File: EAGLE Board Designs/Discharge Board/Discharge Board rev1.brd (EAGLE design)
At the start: 59 x 77 mm, 25 parts, among them J100 CONNECTOR-2_MICROFIT_SMD_RIGH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, J101 CONNECTOR-2_MICROFIT_SMD_RIGH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, K1 RELAY_SPST_NC_POLARIZED_D_24

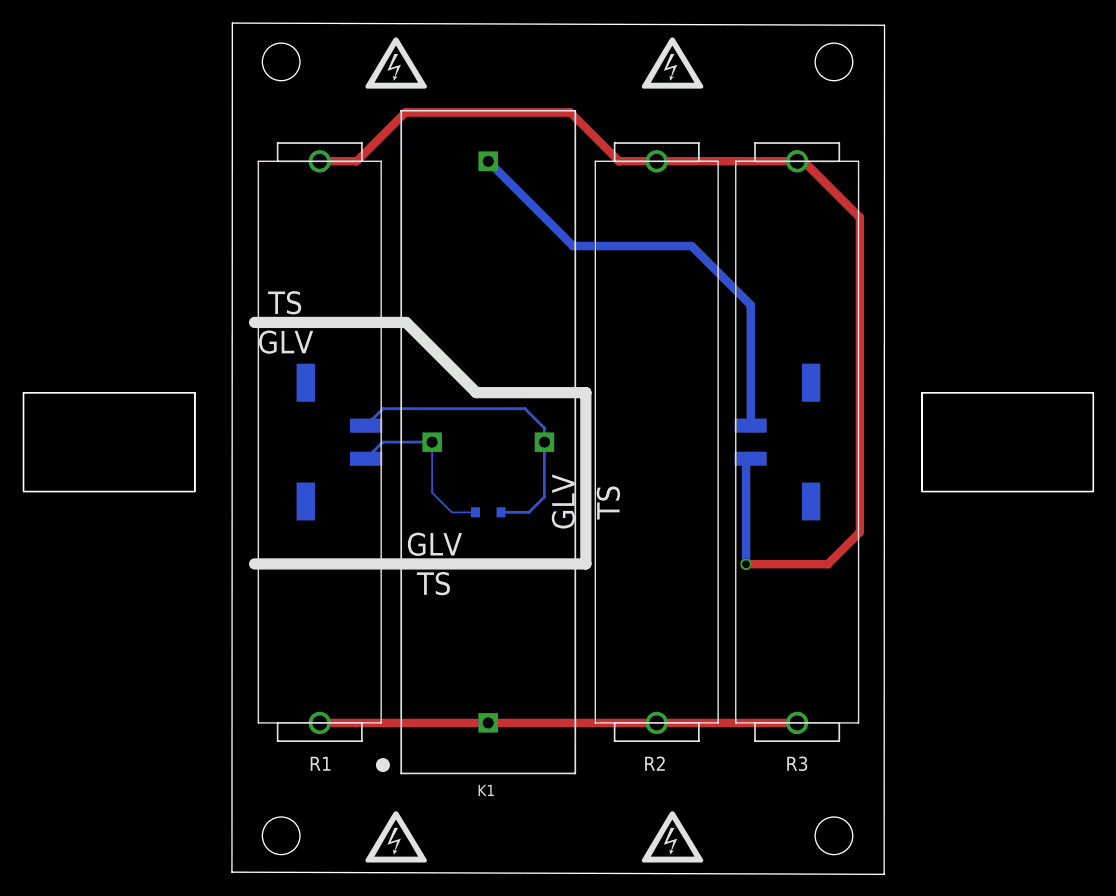
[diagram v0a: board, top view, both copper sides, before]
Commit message: passed review
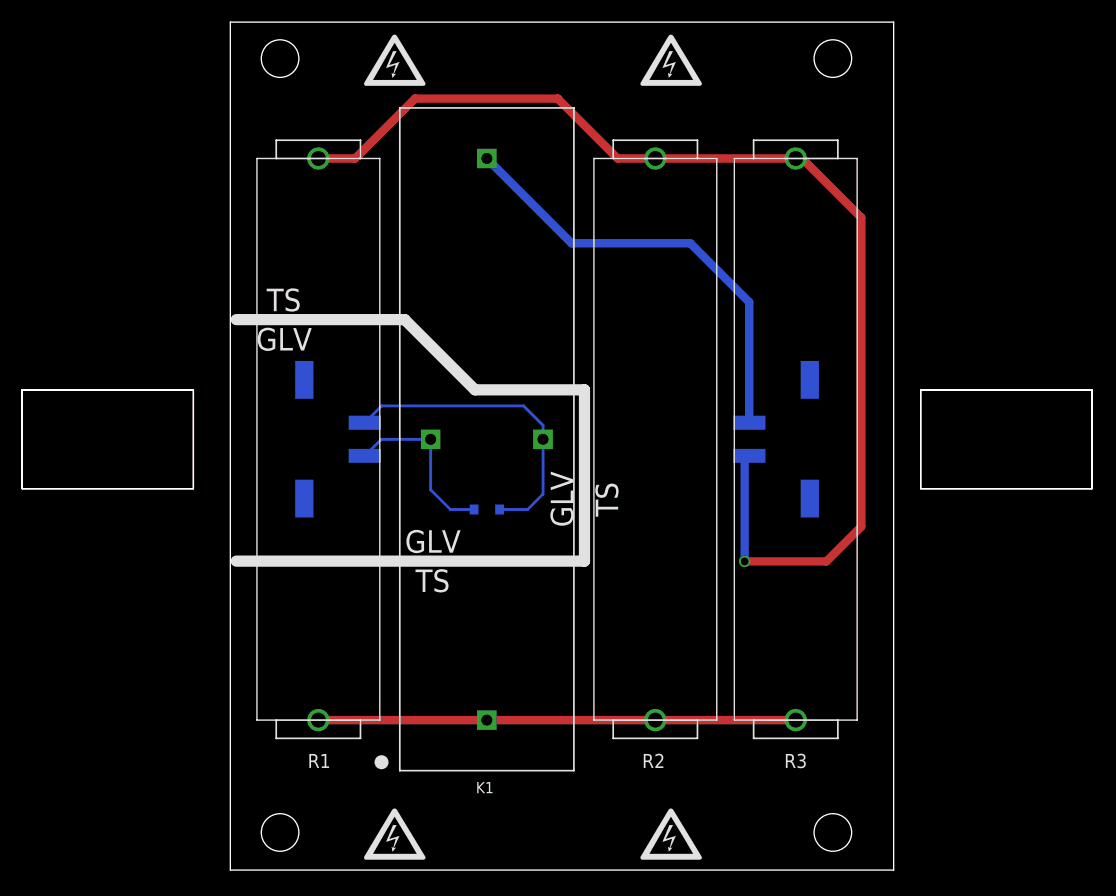
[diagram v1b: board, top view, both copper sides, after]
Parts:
- moved U$18 0.32 mm to (54.5, 73.4)
- moved U$17 0.32 mm to (4.50, 73.4)
- moved U$16 0.32 mm to (54.5, 3.40)
- moved U$15 0.32 mm to (4.50, 3.40)
- moved U$10 0.28 mm to (39.9, 73.3)
- moved U$11 0.28 mm to (39.9, 73.3)
- moved U$6 0.28 mm to (34.1, 33.5)
- moved U$12 0.28 mm to (14.9, 73.3)
- moved U$8 0.28 mm to (14.9, 73.3)
- moved U$3 0.28 mm to (4.86, 51.6)
- moved D100 0.28 mm to (23.2, 32.6)
- moved U$5 0.28 mm to (30.0, 33.5)
- moved U$13 0.28 mm to (39.9, 3.25)
- moved U$9 0.28 mm to (39.9, 3.25)
- moved U$2 0.28 mm to (18.3, 29.7)
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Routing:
- net N$5: track 104.3 -> 105.3 mm
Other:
- board size 59 x 77 mm -> 60 x 76.7 mm
- board text added: "HyTech Racing 2023 Discharge Board rev1 Designed by Zheng-Yin Lee"
- board text removed: "HyTech Racing 2023 Discharge Board Designed by Zheng-Yin Lee"

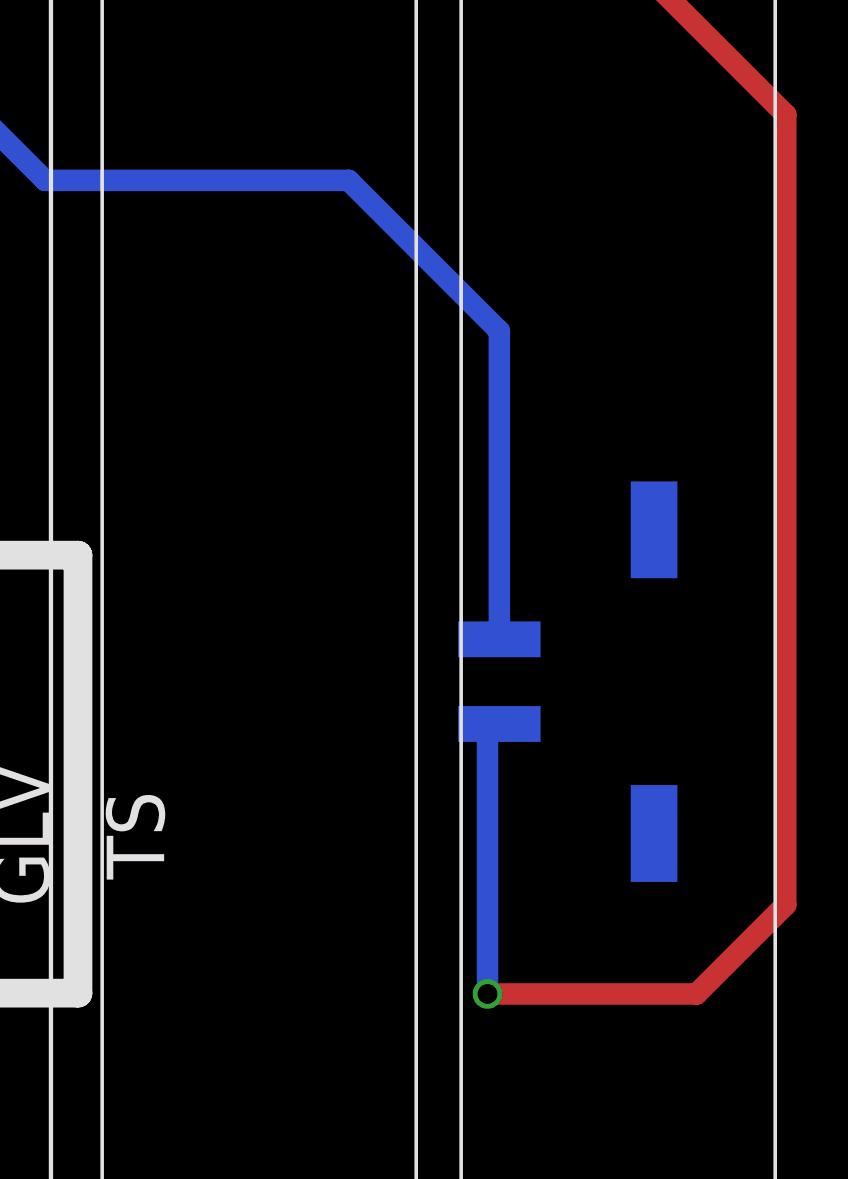
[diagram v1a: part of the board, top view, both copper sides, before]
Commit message: exported
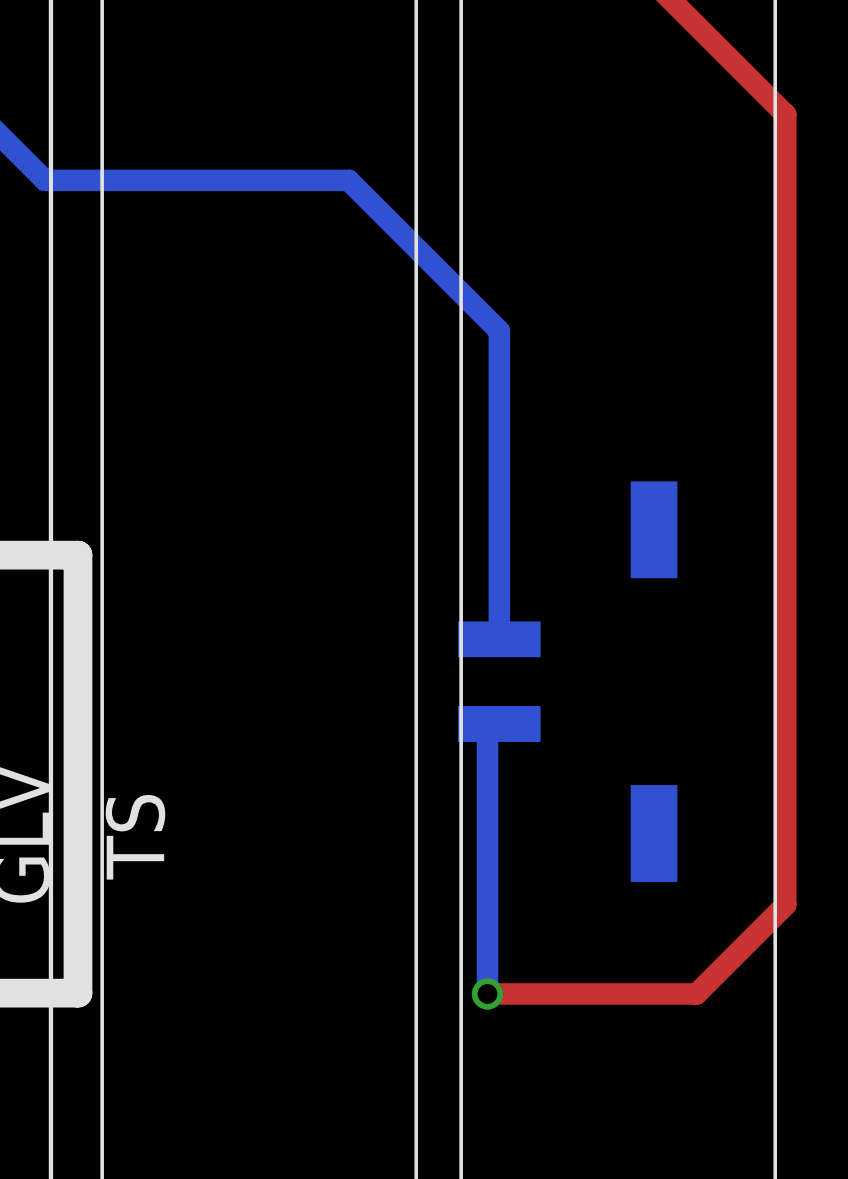
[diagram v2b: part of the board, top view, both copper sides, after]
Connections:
- net N$5 renamed TS-UNFUSED
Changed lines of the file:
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@@
 <setting verticaltext="up"/>
 </settings>
-<grid distance="1" unitdist="mm" unit="mm" style="lines" multiple="1" display="no" altdistance="5" altunitdist="mil" altunit="mil"/>
+<grid distance="30" unitdist="mil" unit="mil" style="lines" multiple="1" display="no" altdistance="5" altunitdist="mil" altunit="mil"/>
 <layers>
 <layer number="1" name="Top" color="4" fill="1" visible="yes" active="yes"/>
@@
 </class>
 </classes>
-<designrules name="JLCPCB (2 Layer)">
-<description language="en">&lt;b&gt;JLCPCB Design Rules (2 Layers)&lt;/b&gt;
+<designrules name="HyTech Default (2 Layer)">
+<description language="en">
+&lt;b&gt;HyTech Default Design Rules (2 Layer)&lt;/b&gt;
 &lt;p&gt;
-The default Design Rules have been set to cover
-a wide range of applications.
-&lt;p&gt;
-Source: &lt;a href=&quot;https://jlcpcb.com/capabilities/Capabilities&quot;&gt;JLCPCB&lt;/a&gt;
-&lt;/p&gt;</description>
+These design rules are designed to pass any PCB fab (JLCPCB, Advanced Circuits, OshPark, Sunstone Circuits) the team uses.
+</description>
 <param name="layerSetup" value="(1*16)"/>
 <param name="mtCopper" value="0.035mm 0.035mm 0.035mm 0.035mm 0.035mm 0.035mm 0.035mm 0.035mm 0.035mm 0.035mm 0.035mm 0.035mm 0.035mm 0.035mm 0.035mm 0.035mm"/>
 <param name="mtIsolate" value="1.53mm 0.15mm 0.2mm 0.15mm 0.2mm 0.15mm 0.2mm 0.15mm 0.2mm 0.15mm 0.2mm 0.15mm 0.2mm 0.15mm 0.2mm"/>
-<param name="mdWireWire" value="5mil"/>
-<param name="mdWirePad" value="5mil"/>
+<param name="mdWireWire" value="6mil"/>
+<param name="mdWirePad" value="6mil"/>
 <param name="mdWireVia" value="8mil"/>
-<param name="mdPadPad" value="5mil"/>
+<param name="mdPadPad" value="6mil"/>
 <param name="mdPadVia" value="10mil"/>
 <param name="mdViaVia" value="20mil"/>
-<param name="mdSmdPad" value="5mil"/>
+<param name="mdSmdPad" value="6mil"/>
 <param name="mdSmdVia" value="10mil"/>
-<param name="mdSmdSmd" value="5mil"/>
-<param name="mdViaViaSameLayer" value="6mil"/>
+<param name="mdSmdSmd" value="6mil"/>
+<param name="mdViaViaSameLayer" value="8mil"/>
 <param name="mnLayersViaInSmd" value="2"/>
-<param name="mdCopperDimension" value="0.2mm"/>
+<param name="mdCopperDimension" value="20mil"/>
 <param name="mdDrill" value="21mil"/>
 <param name="mdSmdStop" value="0mil"/>
-<param name="msWidth" value="5mil"/>
-<param name="msDrill" value="0.3mm"/>
+<param name="msWidth" value="6mil"/>
+<param name="msDrill" value="14mil"/>
 <param name="msMicroVia" value="9.99mm"/>
 <param name="msBlindViaRatio" value="0.5"/>
@@
 <param name="rvViaOuter" value="0.25"/>
 <param name="rvViaInner" value="0.25"/>
-<param name="rvMicroViaOuter" value="0"/>
-<param name="rvMicroViaInner" value="0"/>
-<param name="rlMinPadTop" value="6mil"/>
+<param name="rvMicroViaOuter" value="0.25"/>
+<param name="rvMicroViaInner" value="0.25"/>
+<param name="rlMinPadTop" value="7mil"/>
 <param name="rlMaxPadTop" value="20mil"/>
-<param name="rlMinPadInner" value="6mil"/>
+<param name="rlMinPadInner" value="7mil"/>
 <param name="rlMaxPadInner" value="20mil"/>
-<param name="rlMinPadBottom" value="6mil"/>
+<param name="rlMinPadBottom" value="8mil"/>
 <param name="rlMaxPadBottom" value="20mil"/>
-<param name="rlMinViaOuter" value="6mil"/>
-<param name="rlMaxViaOuter" value="12mil"/>
-<param name="rlMinViaInner" value="6mil"/>
-<param name="rlMaxViaInner" value="12mil"/>
-<param name="rlMinMicroViaOuter" value="6mil"/>
+<param name="rlMinViaOuter" value="8mil"/>
+<param name="rlMaxViaOuter" value="20mil"/>
+<param name="rlMinViaInner" value="8mil"/>
+<param name="rlMaxViaInner" value="20mil"/>
+<param name="rlMinMicroViaOuter" value="8mil"/>
 <param name="rlMaxMicroViaOuter" value="20mil"/>
-<param name="rlMinMicroViaInner" value="6mil"/>
+<param name="rlMinMicroViaInner" value="8mil"/>
 <param name="rlMaxMicroViaInner" value="20mil"/>
 <param name="psTop" value="-1"/>
@@
 <contactref element="K1" pad="2"/>
 <contactref element="J100" pad="2"/>
-<wire x1="46.7107" y1="40.2344" x2="46.9393" y2="40.463" width="0.1524" layer="16"/>
 <wire x1="23.203" y1="64.3644" x2="30.8702" y2="56.6972" width="0.762" layer="16"/>
 <wire x1="30.8702" y1="56.6972" x2="41.6088" y2="56.6972" width="0.762" layer="16"/>
-<wire x1="46.9393" y1="51.3667" x2="41.6088" y2="56.6972" width="0.762" layer="16"/>
-<wire x1="46.9393" y1="40.463" x2="46.9393" y2="51.3667" width="0.762" layer="16"/>
+<wire x1="41.6088" y1="56.6972" x2="46.867" y2="51.439" width="0.762" layer="16"/>
+<wire x1="46.867" y1="51.439" x2="46.9393" y2="51.3667" width="0.762" layer="16"/>
+<wire x1="46.9393" y1="51.3667" x2="46.9393" y2="40.463" width="0.762" layer="16"/>
 </signal>
 <signal name="N$51">
@@
 <wire x1="38.443" y1="13.5644" x2="51.143" y2="13.5644" width="0.762" layer="1"/>
 </signal>
-<signal name="N$5">
+<signal name="TS-UNFUSED">
 <contactref element="R1" pad="1"/>
 <contactref element="R2" pad="1"/>
